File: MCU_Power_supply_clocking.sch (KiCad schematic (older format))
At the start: 114 parts, among them U6 STM32H743ZIT6, Y2 NX5032GA-8MHz, Y3 NX3215SA-32.768K-STD-MUA-14

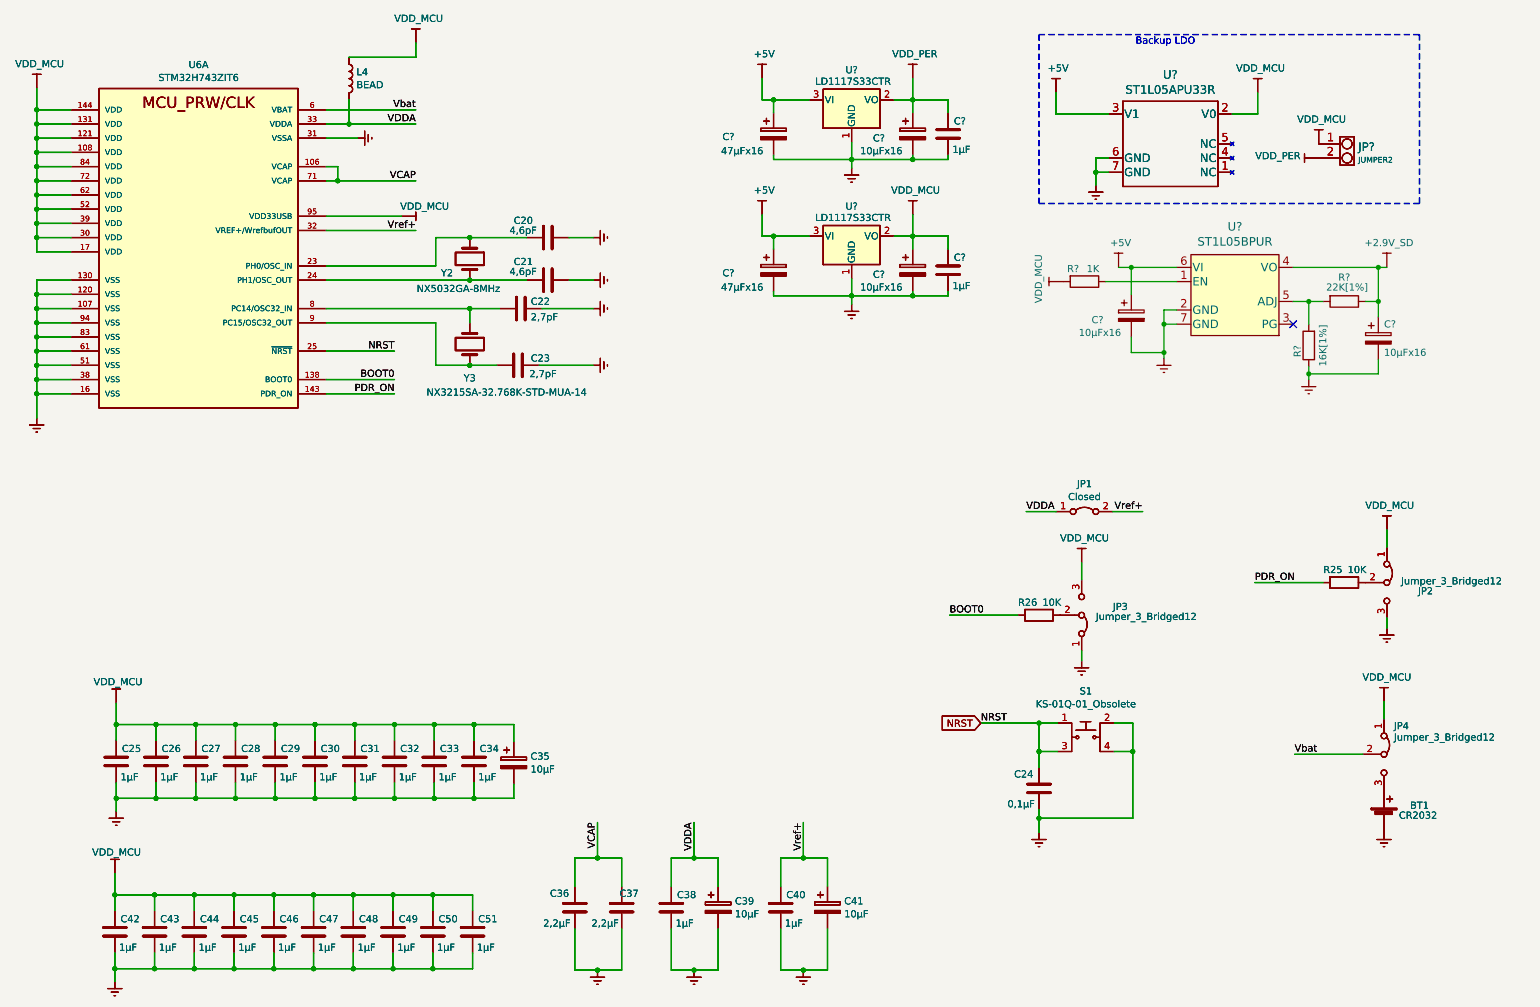
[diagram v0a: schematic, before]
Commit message: start create Analog IO
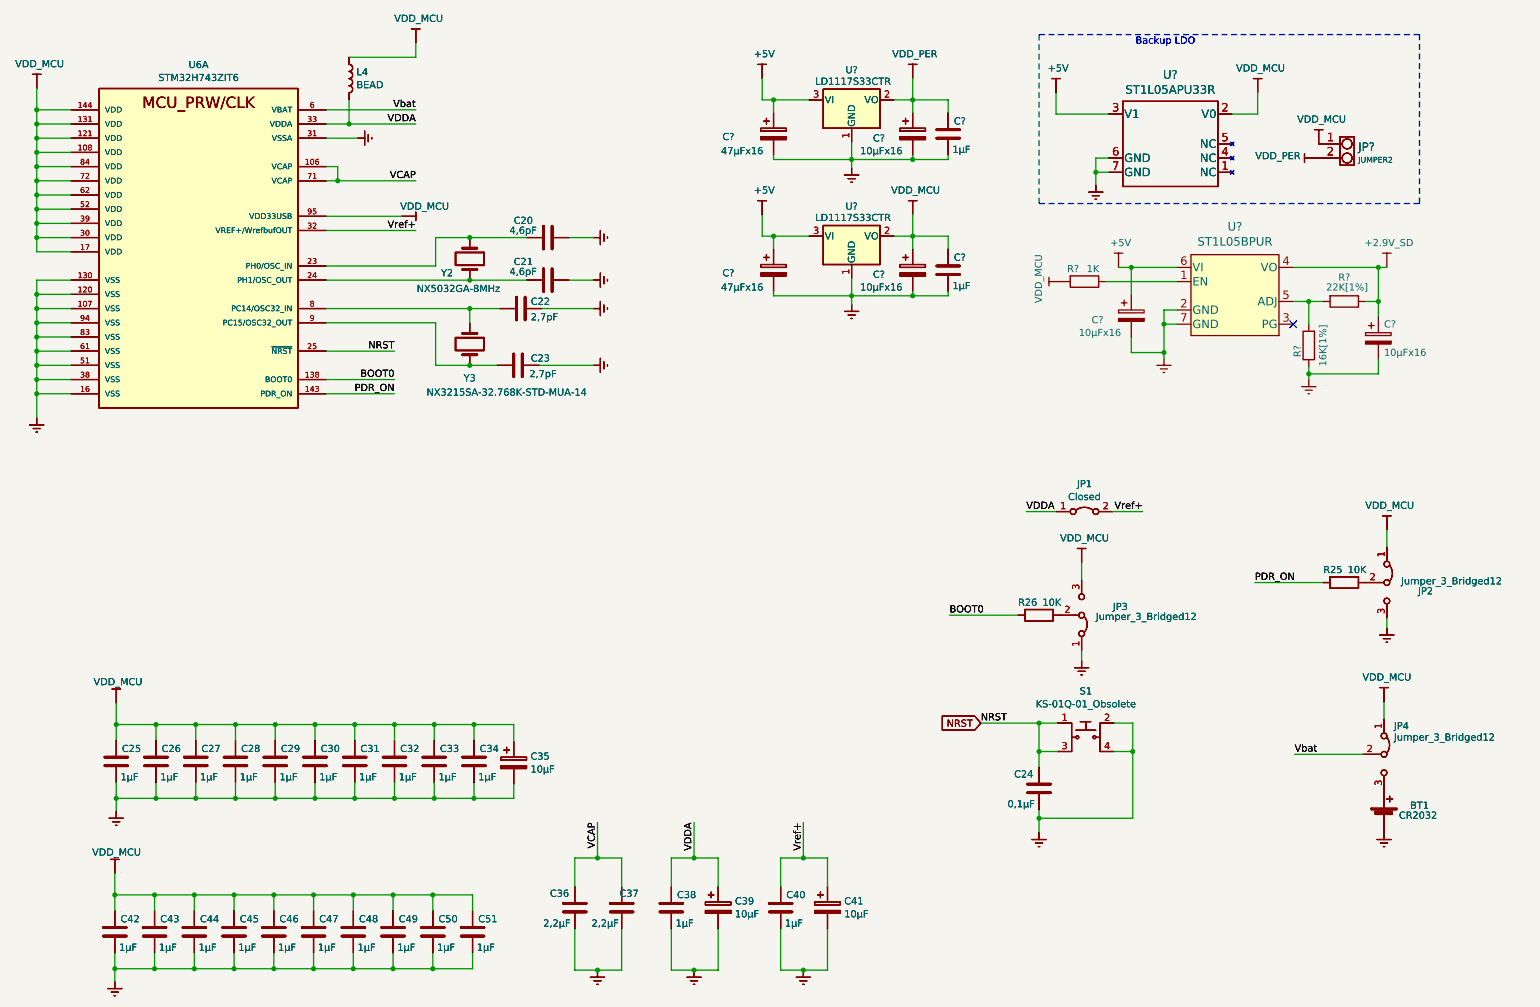
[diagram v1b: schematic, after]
